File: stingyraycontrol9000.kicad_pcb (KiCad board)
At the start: 2 copper layers, 12 parts, among them J1 Screw_Terminal_01x04, J2 Screw_Terminal_01x04, J3 Screw_Terminal_01x02, J4 Conn_01x04, U1 ws2801, U2 LDD-L, U3 LDD-H

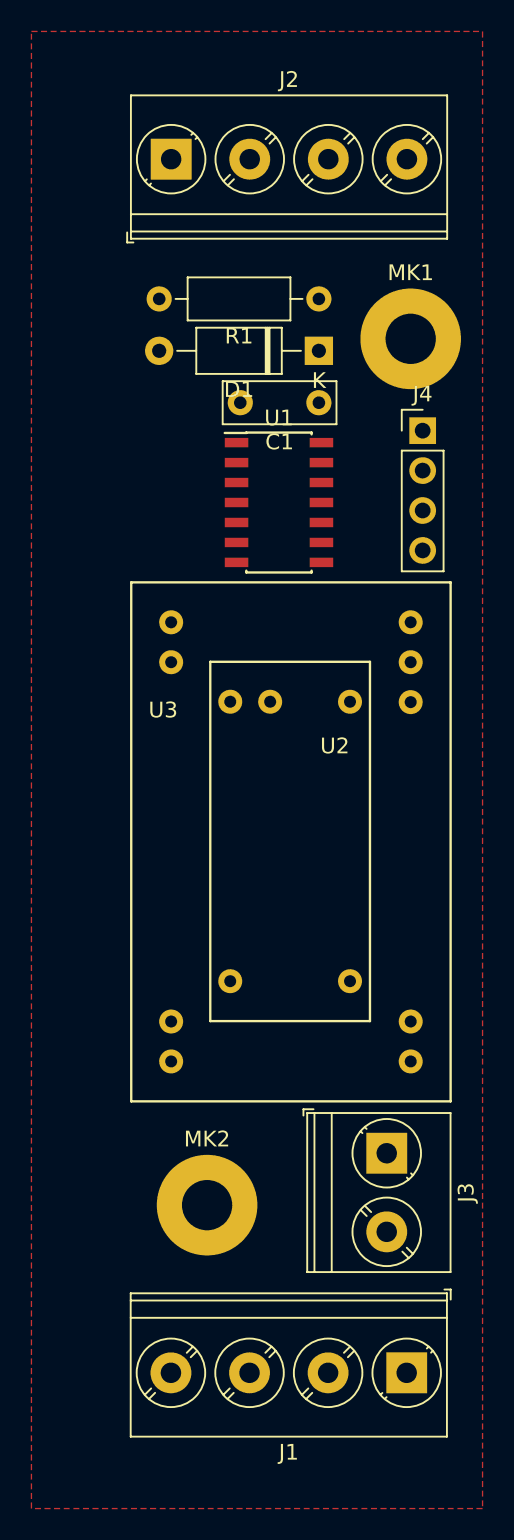
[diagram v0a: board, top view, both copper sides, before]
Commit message: route board
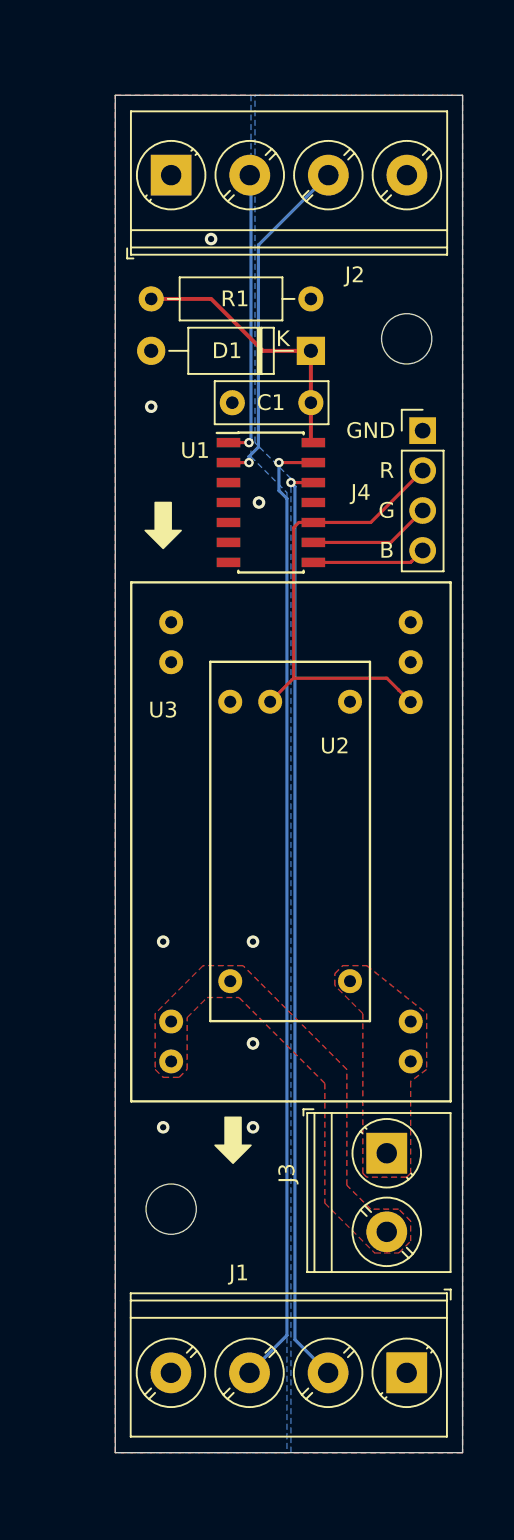
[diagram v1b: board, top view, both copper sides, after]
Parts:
- MK1, MK2: footprint MountingHole:MountingHole_3.2mm_M3_Pad -> MountingHole:MountingHole_3.2mm_M3
- moved MK2 2.30 mm to (130.0, 135.9)
- moved J2 1.02 mm to (130.0, 70.1)
- moved C1 0.51 mm to (138.9, 84.6)
- moved D1 0.51 mm to (138.9, 81.3)
- moved R1 0.51 mm to (138.9, 78.0)
- moved U1 0.51 mm to (136.4, 90.9)
- moved MK1 0.25 mm to (145.0, 80.5)
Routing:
- net /CKO: track 0.00 -> 61.3 mm, vias 0 -> 1
- net /SDO: track 0.00 -> 59.1 mm, vias 0 -> 1
- net /ROUT: track 0.00 -> 29.5 mm
- net /SDI: track 0.00 -> 21.7 mm, vias 0 -> 1
- net /CKI: track 0.00 -> 18.4 mm, vias 0 -> 1
- net +5V: track 0.00 -> 17.4 mm
- net /GOUT: track 0.00 -> 7.79 mm
- net /BOUT: track 0.00 -> 7.27 mm
- net GND: vias 0 -> 8
- added copper zone on B.Cu, net +24V
- added copper zone on F.Cu, net /LED+
- added copper zone on F.Cu, net /LED-
- added copper zone on B.Cu, net GND
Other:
- board outline added: 22.1 x 86.4 mm
- net class Default: trace_width 0.25 -> 0.2
- net class data added: clearance 0.2, trace_width 0.2, via_dia 0.6, via_drill 0.3
- net class power added: clearance 0.2, trace_width 0.25, via_dia 0.8, via_drill 0.4
- board text added: "B"
- board text added: "CKI"
- board text added: "CKO"
- board text added: "G"
- board text added: "GND"
- board text added: "LED+"
- board text added: "LED-"
- board text added: "R"
- board text added: "SDI"
- board text added: "SDO"
- board text added: "VCC"
- board text added: "stingyraycontrol9000"
